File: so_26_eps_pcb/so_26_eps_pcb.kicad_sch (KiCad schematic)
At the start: 8 parts, among them U1 LM22679TJ-ADJ/NOPB

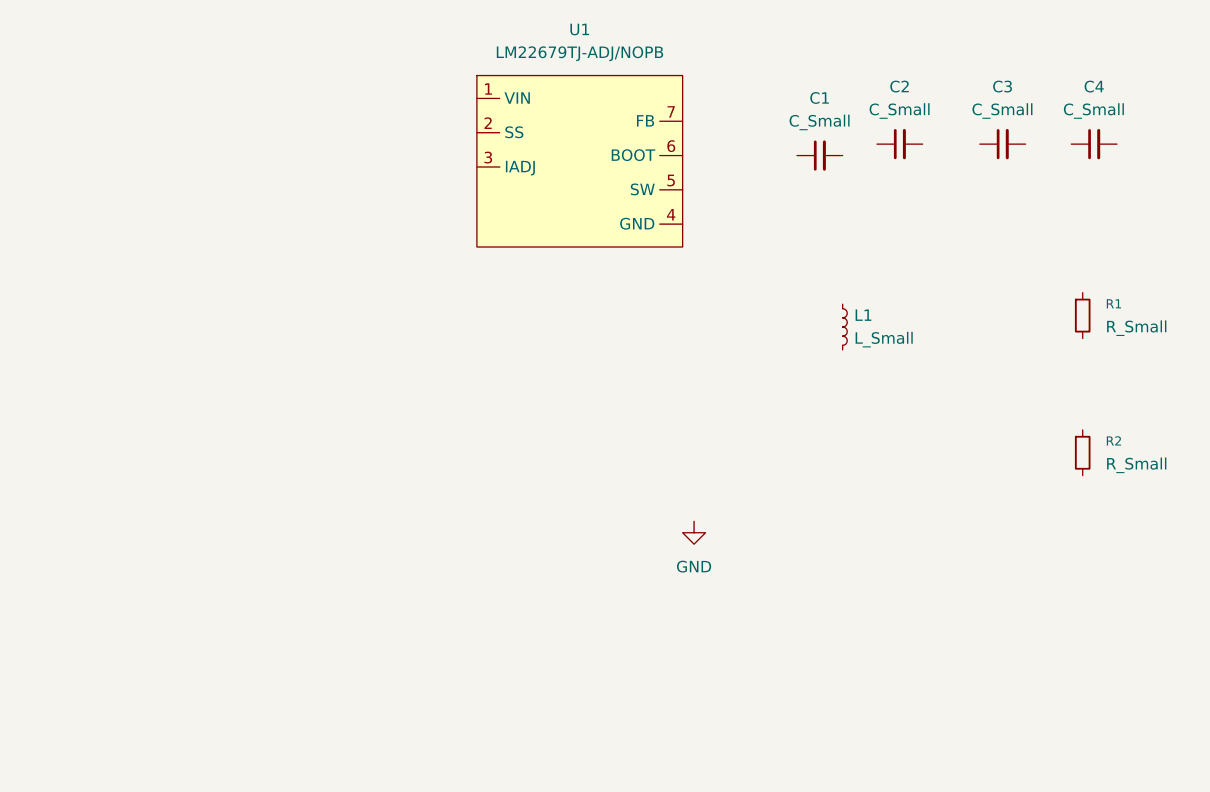
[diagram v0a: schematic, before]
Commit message: Battery
Yuhhh
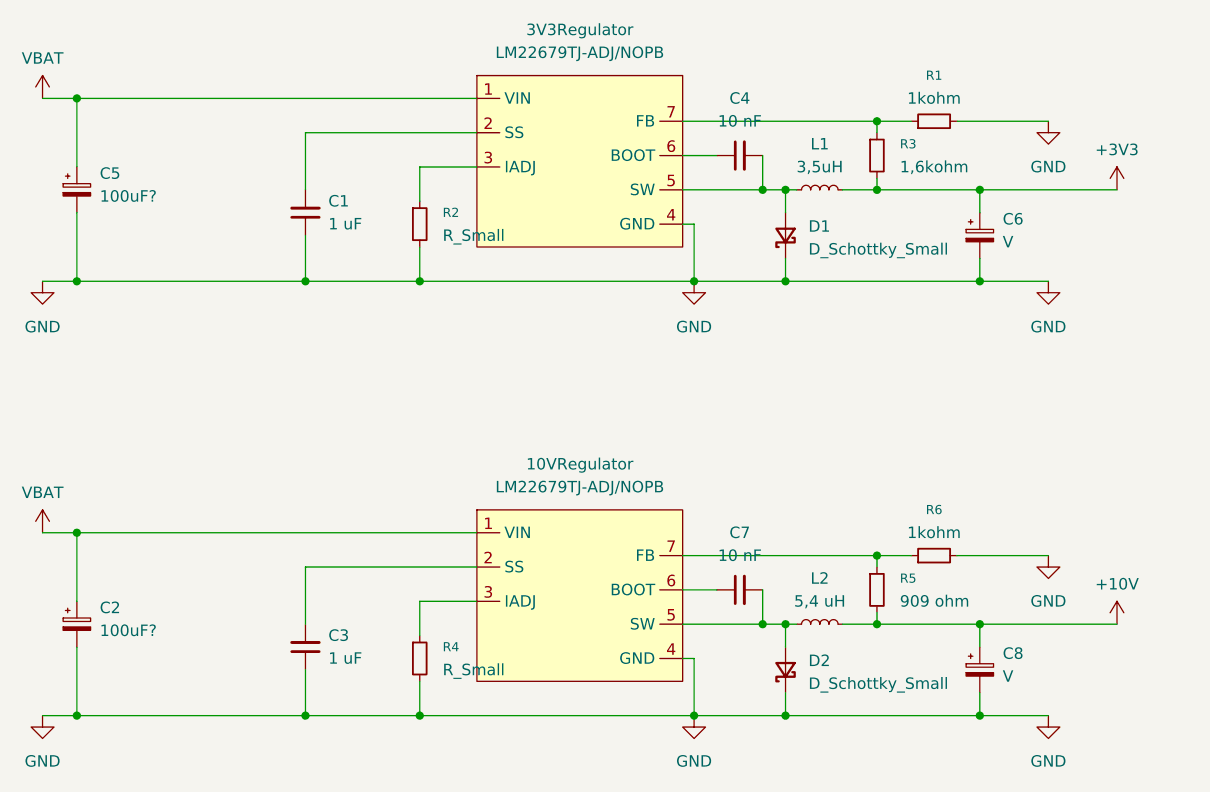
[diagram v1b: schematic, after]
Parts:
- removed C2: C_Small, symbol Device:C_Small
- added 10VRegulator: LM22679TJ-ADJ/NOPB, symbol MySymbols:LM22679TJ-ADJ/NOPB
- added C2, C5: 100uF?, symbol Device:C_Polarized_Small
- added C6, C8: V, symbol Device:C_Polarized_Small
- added C7: 10 nF, symbol Device:C_Small
- added D1, D2: D_Schottky_Small, symbol Device:D_Schottky_Small
- added L2: 5,4 uH, symbol Device:L_Small
- added R3: 1,6kohm, symbol Device:R_Small
- added R4: R_Small, symbol Device:R_Small
- added R5: 909 ohm, symbol Device:R_Small
- added R6: 1kohm, symbol Device:R_Small
- C1, C3: value C_Small -> 1 uF
- C4: value C_Small -> 10 nF
- L1: value L_Small -> 3,5uH
- R1: value R_Small -> 1kohm
- renumbered U1 to 3V3Regulator
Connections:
- net GND: now also 3V3Regulator.4 (GND), C1.1, C3.1, R1.2, R2.2, 10VRegulator.4 (GND), C2.2, C5.2, C6.2, C8.2, D1.1 (K), D2.1 (K), R4.2, R6.2
- net at C1.2: now also 3V3Regulator.2 (SS)
- net at L1.1: now also 3V3Regulator.5 (SW), C4.2, D1.2 (A)
- net +3V3: now reaches L1.2
- net +3V3: now also C6.1, R3.2
- net at R2.1: now also 3V3Regulator.3 (IADJ)
- net at C4.1: now also 3V3Regulator.6 (BOOT)
- net at R1.1: now also 3V3Regulator.7 (FB), R3.1
- net at C3.2: now also 10VRegulator.2 (SS)
- net VBAT: now reaches 3V3Regulator.1 (VIN)
- net VBAT: now also 10VRegulator.1 (VIN), C2.1, C5.1
- new net: 10VRegulator.7 (FB), R5.1, R6.1
- new net: 10VRegulator.5 (SW), C7.2, D2.2 (A), L2.1
- new net: 10VRegulator.3 (IADJ), R4.1
- new net: 10VRegulator.6 (BOOT), C7.1
- new net +10V: C8.1, L2.2, R5.2
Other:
- moved on the sheet: C1, C4, L1, R1, R2
